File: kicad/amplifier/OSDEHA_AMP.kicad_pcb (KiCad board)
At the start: 2 copper layers, 89 parts, among them J1 INPUT, J2 HEATERS DC, J3 PSU HV, J4 OUTPUT, J5 DHT FIL2, J6 DHT FIL1, Q1 DN2540N5-G, Q10 DN2540, Q2 DN2540N5-G, Q3 STF3LN80K5, Q4 STF3LN80K5, Q5 AOT1N60, Q6 IXTP3N100D2, Q7 AOT1N60, Q8 IXTP3N100D2, Q9 DN2540, SW1 SW_DPDT_x2, U1 6E5P, U2 6E5P, U3 801A, U4 801A

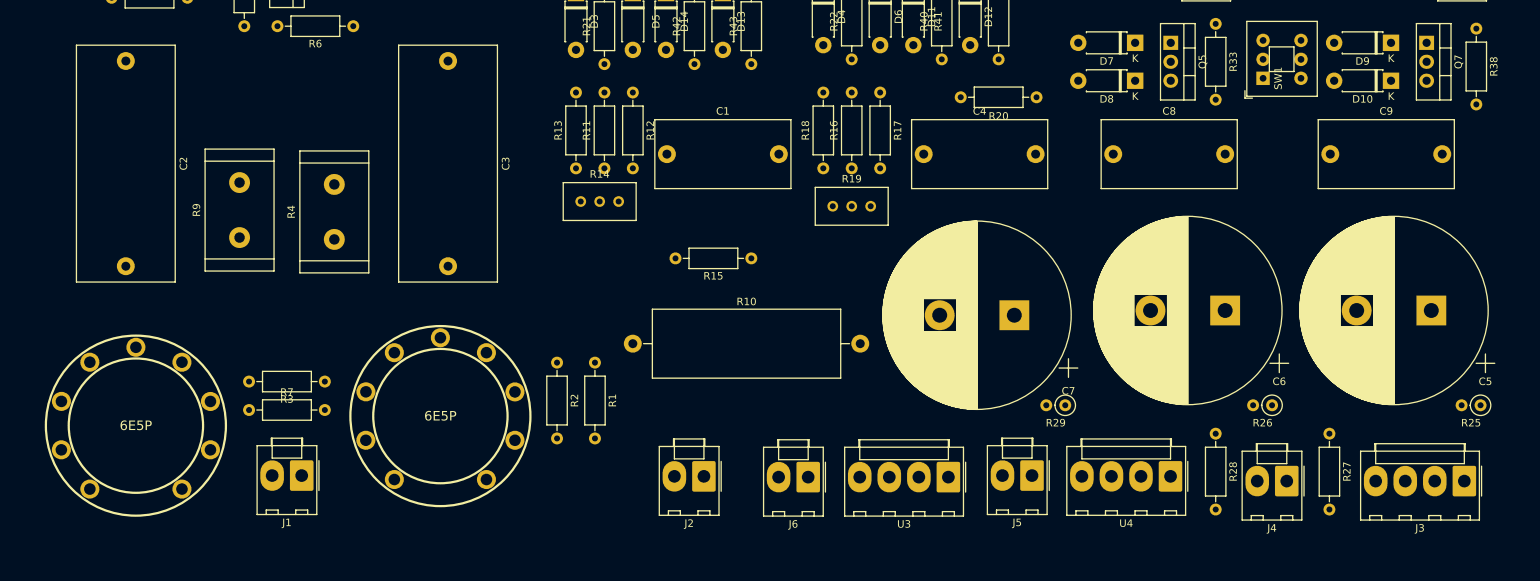
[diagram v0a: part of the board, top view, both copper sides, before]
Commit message: up
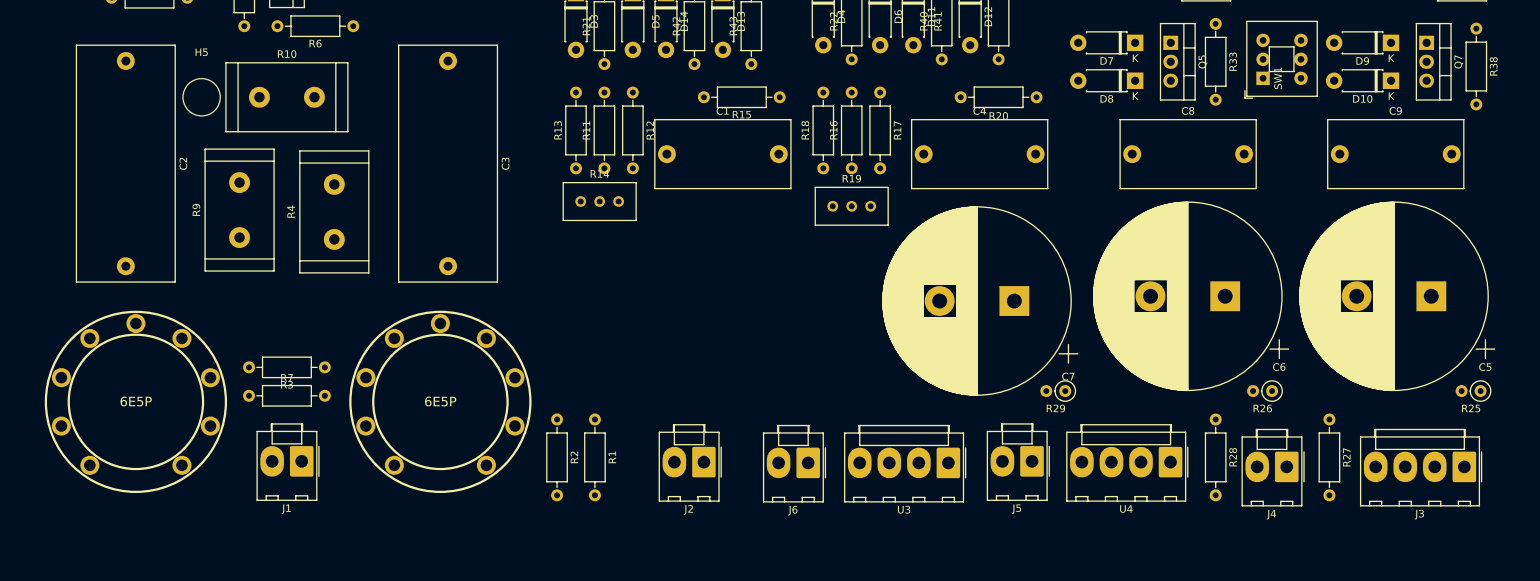
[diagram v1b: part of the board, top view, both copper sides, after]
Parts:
- added H5: VENTILATION, MountingHole:MountingHole_5mm, F.Cu at (-30.5, 39.4)
- R10: footprint Resistor_THT:R_Axial_Power_L25.0mm_W9.0mm_P30.48mm -> Resistor_THT:R_Radial_Power_L16.1mm_W9.0mm_P7.37mm
- moved R10 59.9 mm to (-22.7, 39.4)
- moved R15 21.9 mm to (47.0, 39.4)
- moved R1 7.62 mm to (22.2, 82.5)
- moved R2 7.62 mm to (17.1, 82.5)
- moved U2 3.19 mm to (-39.3, 80.2)
- moved C8 2.54 mm to (94.2, 47.0)
- moved C7 1.91 mm to (78.4, 66.7)
- moved J1 1.91 mm to (-17.1, 88.2)
- moved J2 1.91 mm to (36.8, 88.3)
- moved J3 1.91 mm to (138.7, 88.9)
- moved J4 1.91 mm to (114.9, 88.9)
- moved J5 1.91 mm to (80.8, 88.2)
- moved J6 1.91 mm to (50.8, 88.4)
- moved R25 1.91 mm to (140.9, 78.7)
- moved R26 1.91 mm to (113.0, 78.7)
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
